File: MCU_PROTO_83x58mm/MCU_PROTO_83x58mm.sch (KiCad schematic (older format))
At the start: 17 parts, among them J1 Screw_Terminal_01x03, J10 Conn_01x20_Female, J11 Conn_01x01_Male, J12 Conn_01x01_Male, J2 Screw_Terminal_01x03, J3 Conn_01x20_Female, J4 Conn_01x20_Female, J5 Conn_01x20_Female, J6 Conn_01x20_Female, J7 Conn_01x20_Female, J8 Conn_01x20_Female, J9 Conn_01x20_Female

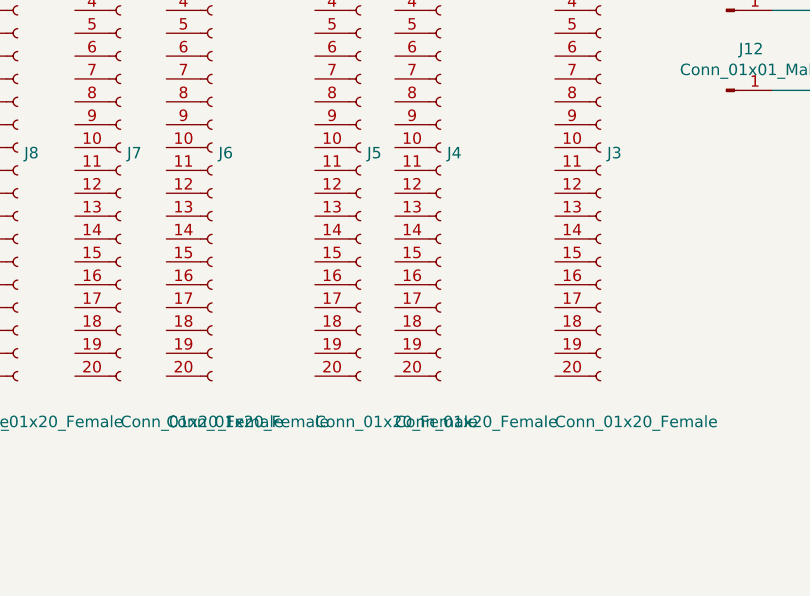
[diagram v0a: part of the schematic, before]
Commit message: gerbers sinlge corrected
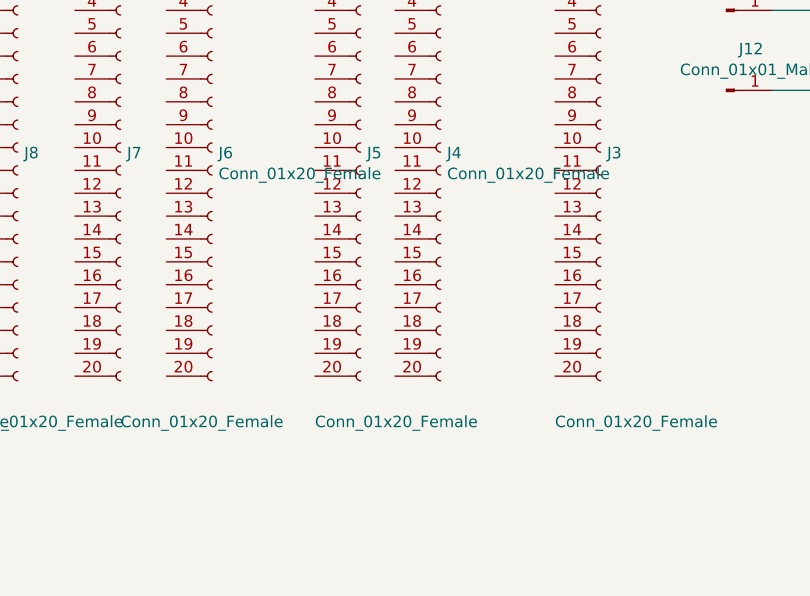
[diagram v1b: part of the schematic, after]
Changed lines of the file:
@@
 Text Notes 4800 1450 0    50   ~ 0
 NANO &\nBLUEPILL
-$Comp
-L Connector:Conn_01x20_Female J6
-U 1 1 61975404
-P 5050 2550
-F 0 "J6" H 5078 2526 50  0000 L CNN
-F 1 "Conn_01x20_Female" H 4850 1350 50  0000 L CNN
-F 2 "Connector_PinSocket_2.54mm:PinSocket_1x20_P2.54mm_Vertical" H 5050 2550 50  0001 C CNN
-F 3 "~" H 5050 2550 50  0001 C CNN
-	1    5050 2550
-	1    0    0    -1
-$EndComp
 Text Notes 4400 1450 0    50   ~ 0
 RPI\nPICO
@@
 $EndComp
 $Comp
-L Connector:Conn_01x20_Female J4
-U 1 1 6217E1D9
-P 6050 2550
-F 0 "J4" H 6078 2526 50  0000 L CNN
-F 1 "Conn_01x20_Female" H 5850 1350 50  0000 L CNN
-F 2 "Connector_PinSocket_2.54mm:PinSocket_1x20_P2.54mm_Vertical" H 6050 2550 50  0001 C CNN
-F 3 "~" H 6050 2550 50  0001 C CNN
-	1    6050 2550
-	1    0    0    -1
-$EndComp
-$Comp
 L Connector:Conn_01x20_Female J5
 U 1 1 620C51CD
@@
 Text Notes 5700 1450 0    50   ~ 0
 RPI\nZERO
+$Comp
+L Connector:Conn_01x20_Female J6
+U 1 1 620D8961
+P 5050 2550
+F 0 "J6" H 5078 2526 50  0000 L CNN
+F 1 "Conn_01x20_Female" H 5078 2435 50  0000 L CNN
+F 2 "Connector_PinSocket_2.54mm:PinSocket_1x20_P2.54mm_Vertical" H 5050 2550 50  0001 C CNN
+F 3 "~" H 5050 2550 50  0001 C CNN
+	1    5050 2550
+	1    0    0    -1
+$EndComp
+$Comp
+L Connector:Conn_01x20_Female J4
+U 1 1 620DD7F6
+P 6050 2550
+F 0 "J4" H 6078 2526 50  0000 L CNN
+F 1 "Conn_01x20_Female" H 6078 2435 50  0000 L CNN
+F 2 "Connector_PinSocket_2.54mm:PinSocket_1x20_P2.54mm_Vertical" H 6050 2550 50  0001 C CNN
+F 3 "~" H 6050 2550 50  0001 C CNN
+	1    6050 2550
+	1    0    0    -1
+$EndComp
 $EndSCHEMATC
